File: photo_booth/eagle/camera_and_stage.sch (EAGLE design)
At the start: 9 parts

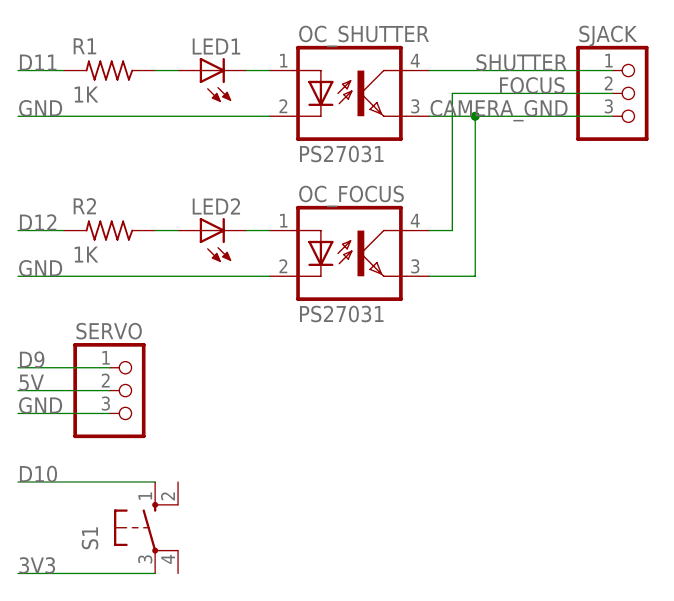
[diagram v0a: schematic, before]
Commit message: LEDはいらない子
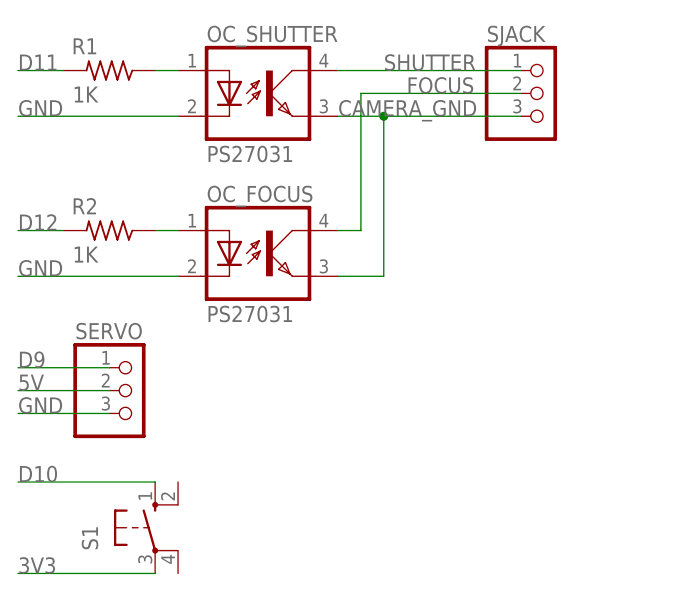
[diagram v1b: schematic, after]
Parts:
- removed LED1, LED2: (no value), led:LED5MM
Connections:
- removed net N$3: LED2.C, OC_FOCUS.A
- removed net N$4: LED1.C, OC_SHUTTER.A
- net N$2: now also OC_FOCUS.A; no longer LED2.A
- net R1: now also OC_SHUTTER.A; no longer LED1.A
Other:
- moved on the sheet: OC_FOCUS, OC_SHUTTER, SJACK
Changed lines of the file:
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@@
 <?xml version="1.0" encoding="utf-8"?>
 <!DOCTYPE eagle SYSTEM "eagle.dtd">
-<eagle version="6.2">
+<eagle version="6.1">
 <drawing>
 <settings>
@@
 </classes>
 <parts>
-<part name="LED1" library="led" deviceset="LED" device="5MM"/>
 <part name="SERVO" library="pinhead" deviceset="PINHD-1X3" device=""/>
 <part name="OC_SHUTTER" library="PS2703" deviceset="PS2703" device="1"/>
@@
 <part name="R2" library="rcl" deviceset="R-US_" device="0204/7" value="1K"/>
 <part name="SJACK" library="pinhead" deviceset="PINHD-1X3" device=""/>
-<part name="LED2" library="led" deviceset="LED" device="5MM"/>
 <part name="S1" library="TACT" deviceset="10-XX" device=""/>
 </parts>
@@
 </plain>
 <instances>
-<instance part="LED1" gate="G$1" x="30.48" y="101.6" rot="R90"/>
 <instance part="SERVO" gate="A" x="22.86" y="66.04"/>
-<instance part="OC_SHUTTER" gate="G$1" x="48.26" y="99.06"/>
-<instance part="OC_FOCUS" gate="G$1" x="48.26" y="81.28"/>
+<instance part="OC_SHUTTER" gate="G$1" x="38.1" y="99.06"/>
+<instance part="OC_FOCUS" gate="G$1" x="38.1" y="81.28"/>
 <instance part="R1" gate="G$1" x="20.32" y="101.6" smashed="yes" rot="R180">
 <attribute name="NAME" x="19.05" y="105.1814" size="1.778" layer="95" rot="R180"/>
@@
 <attribute name="VALUE" x="19.05" y="82.042" size="1.778" layer="96" rot="R180"/>
 </instance>
-<instance part="SJACK" gate="A" x="78.74" y="99.06"/>
-<instance part="LED2" gate="G$1" x="30.48" y="83.82" rot="R90"/>
+<instance part="SJACK" gate="A" x="68.58" y="99.06"/>
 <instance part="S1" gate="1" x="25.4" y="50.8"/>
 </instances>
@@
 <segment>
 <pinref part="OC_SHUTTER" gate="G$1" pin="C"/>
-<wire x1="38.1" y1="96.52" x2="10.16" y2="96.52" width="0.1524" layer="91"/>
+<wire x1="27.94" y1="96.52" x2="10.16" y2="96.52" width="0.1524" layer="91"/>
 <label x="10.16" y="96.52" size="1.778" layer="95"/>
 </segment>
 <segment>
 <pinref part="OC_FOCUS" gate="G$1" pin="C"/>
-<wire x1="38.1" y1="78.74" x2="10.16" y2="78.74" width="0.1524" layer="91"/>
+<wire x1="27.94" y1="78.74" x2="10.16" y2="78.74" width="0.1524" layer="91"/>
 <label x="10.16" y="78.74" size="1.778" layer="95"/>
 </segment>
@@
 <pinref part="SJACK" gate="A" pin="3"/>
 <pinref part="OC_SHUTTER" gate="G$1" pin="EMIT"/>
-<wire x1="76.2" y1="96.52" x2="60.96" y2="96.52" width="0.1524" layer="91"/>
-<wire x1="60.96" y1="96.52" x2="55.88" y2="96.52" width="0.1524" layer="91"/>
-<wire x1="60.96" y1="78.74" x2="60.96" y2="96.52" width="0.1524" layer="91"/>
-<junction x="60.96" y="96.52"/>
+<wire x1="66.04" y1="96.52" x2="50.8" y2="96.52" width="0.1524" layer="91"/>
+<wire x1="50.8" y1="96.52" x2="45.72" y2="96.52" width="0.1524" layer="91"/>
+<wire x1="50.8" y1="78.74" x2="50.8" y2="96.52" width="0.1524" layer="91"/>
+<junction x="50.8" y="96.52"/>
 <pinref part="OC_FOCUS" gate="G$1" pin="EMIT"/>
-<wire x1="60.96" y1="78.74" x2="55.88" y2="78.74" width="0.1524" layer="91"/>
-<label x="55.88" y="96.52" size="1.778" layer="95"/>
+<wire x1="50.8" y1="78.74" x2="45.72" y2="78.74" width="0.1524" layer="91"/>
+<label x="45.72" y="96.52" size="1.778" layer="95"/>
 </segment>
 </net>
@@
 <pinref part="SJACK" gate="A" pin="1"/>
 <pinref part="OC_SHUTTER" gate="G$1" pin="COL"/>
-<wire x1="76.2" y1="101.6" x2="55.88" y2="101.6" width="0.1524" layer="91"/>
-<label x="60.96" y="101.6" size="1.778" layer="95"/>
+<wire x1="66.04" y1="101.6" x2="45.72" y2="101.6" width="0.1524" layer="91"/>
+<label x="50.8" y="101.6" size="1.778" layer="95"/>
 </segment>
 </net>
@@
 <segment>
 <pinref part="OC_FOCUS" gate="G$1" pin="COL"/>
-<wire x1="58.42" y1="83.82" x2="55.88" y2="83.82" width="0.1524" layer="91"/>
-<wire x1="58.42" y1="83.82" x2="58.42" y2="99.06" width="0.1524" layer="91"/>
+<wire x1="48.26" y1="83.82" x2="45.72" y2="83.82" width="0.1524" layer="91"/>
+<wire x1="48.26" y1="83.82" x2="48.26" y2="99.06" width="0.1524" layer="91"/>
 <pinref part="SJACK" gate="A" pin="2"/>
-<wire x1="58.42" y1="99.06" x2="76.2" y2="99.06" width="0.1524" layer="91"/>
-<label x="63.5" y="99.06" size="1.778" layer="95"/>
+<wire x1="48.26" y1="99.06" x2="66.04" y2="99.06" width="0.1524" layer="91"/>
+<label x="53.34" y="99.06" size="1.778" layer="95"/>
 </segment>
 </net>
 <net name="R1" class="0">
 <segment>
-<pinref part="LED1" gate="G$1" pin="A"/>
 <pinref part="R1" gate="G$1" pin="1"/>
 <wire x1="27.94" y1="101.6" x2="25.4" y2="101.6" width="0.1524" layer="91"/>
+<pinref part="OC_SHUTTER" gate="G$1" pin="A"/>
 </segment>
 </net>
@@
 <segment>
 <pinref part="R2" gate="G$1" pin="1"/>
-<pinref part="LED2" gate="G$1" pin="A"/>
 <wire x1="25.4" y1="83.82" x2="27.94" y2="83.82" width="0.1524" layer="91"/>
+<pinref part="OC_FOCUS" gate="G$1" pin="A"/>
 </segment>
 </net>
-<net name="N$3" class="0">
-<segment>
-<pinref part="LED2" gate="G$1" pin="C"/>
-<pinref part="OC_FOCUS" gate="G$1" pin="A"/>
-<wire x1="35.56" y1="83.82" x2="38.1" y2="83.82" width="0.1524" layer="91"/>
-</segment>
-</net>
-<net name="N$4" class="0">
-<segment>
-<pinref part="OC_SHUTTER" gate="G$1" pin="A"/>
-<pinref part="LED1" gate="G$1" pin="C"/>
-<wire x1="38.1" y1="101.6" x2="35.56" y2="101.6" width="0.1524" layer="91"/>
-</segment>
-</net>
